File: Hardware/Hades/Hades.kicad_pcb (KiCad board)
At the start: 4 copper layers, 100.1 x 60.2 mm, 215 parts, among them SW1 SKRPANE010, SW2 TDD01H0SB1R, SW3 TDD01H0SB1R, SW4 TDD01H0SB1R, SW5 SKRPANE010, U1 INA219AIDCNR, U10 u-blox MAX-8Q, U11 otter:CH330, U12 otter:CH330, U2 PCA9685PW, U3 24CW1280T-I_OT, U4 W25N01GVZEIG_TR, U5 BMI088, U6 TMP100, U7 MPRLS0025PA00001A, U8 IIS2MDCTR, U9 24CW1280T-I_OT

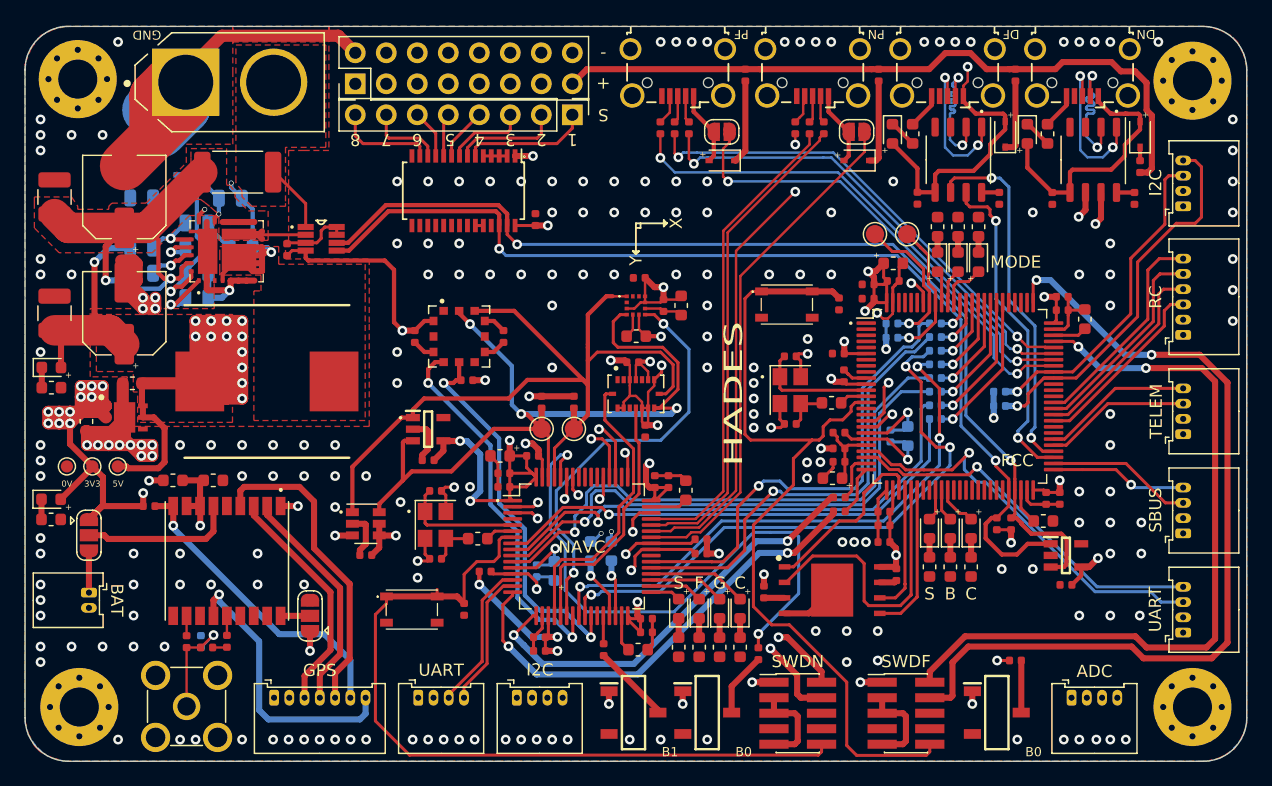
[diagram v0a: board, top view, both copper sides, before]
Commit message: Saved with Kicad 9.0
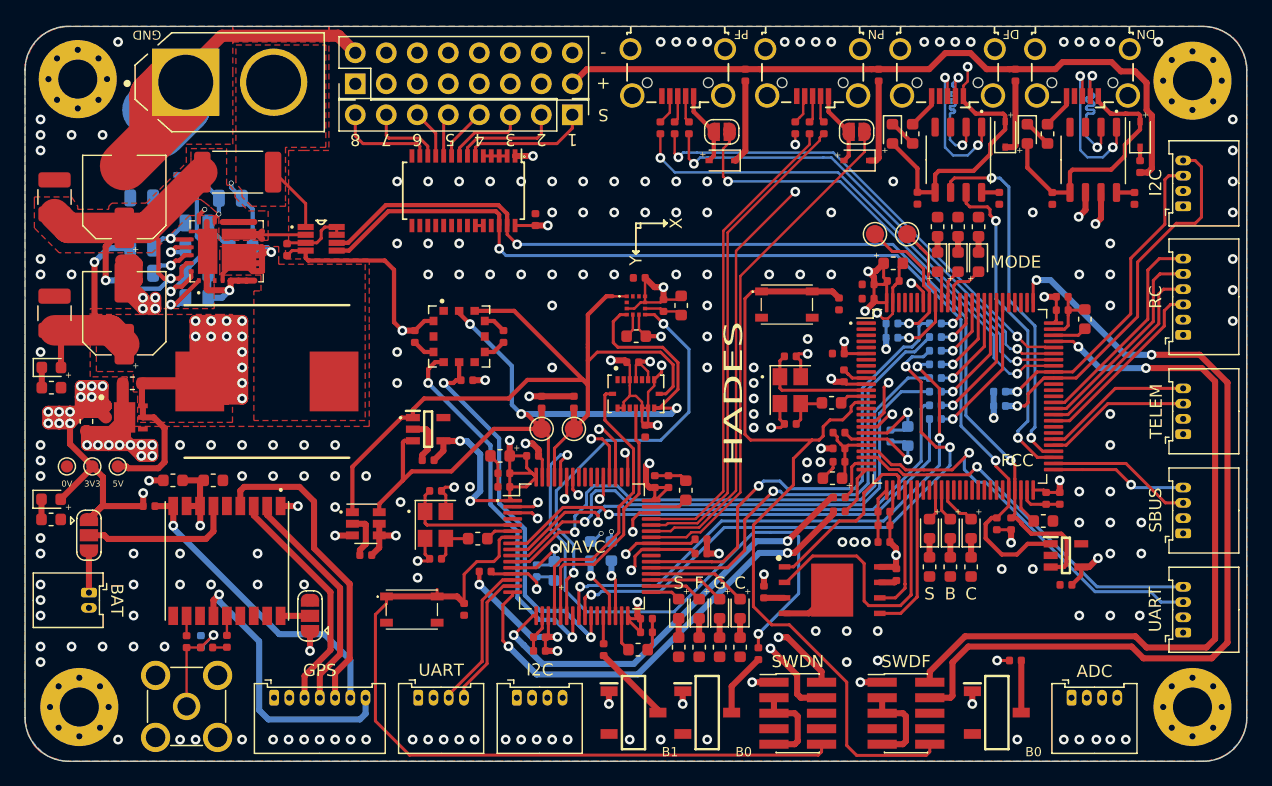
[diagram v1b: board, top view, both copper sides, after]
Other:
- net class Default removed
